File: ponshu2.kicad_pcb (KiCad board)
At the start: 2 copper layers, 61.6 x 41.7 mm, 58 parts, among them J1 Conn_01x04, J10 Conn_01x01, J11 Conn_01x01, J12 Conn_01x01, J13 Conn_01x01, J14 Conn_01x01, J15 Conn_01x01, J16 Conn_01x01, J17 Conn_01x01, J18 Conn_01x01, J19 Conn_01x01, J2 Conn_01x01, J20 Conn_01x01, J21 Conn_01x01, J22 Conn_01x01, J23 Conn_01x01, J24 Conn_01x01, J25 Conn_01x01, J26 Conn_01x01, J27 Conn_01x02, J28 Conn_01x03, J29 Conn_01x01, J3 Conn_01x01, J30 Conn_01x01, J31 Conn_01x01, J32 Conn_01x01, J33 Conn_01x01, J34 Conn_01x01, J35 Conn_01x01, J36 Conn_01x01, J37 Conn_01x01, J38 Conn_01x01, J39 Conn_01x01, J4 Conn_01x01, J5 Conn_01x01, J6 Conn_01x01, J7 Conn_01x01, J8 Conn_01x01, J9 Conn_01x01, SW1 TS-1187A-B-A-B, SW2 TS-1187A-B-A-B, U1 XC6206P332MR, U2 STM32F072CBT6

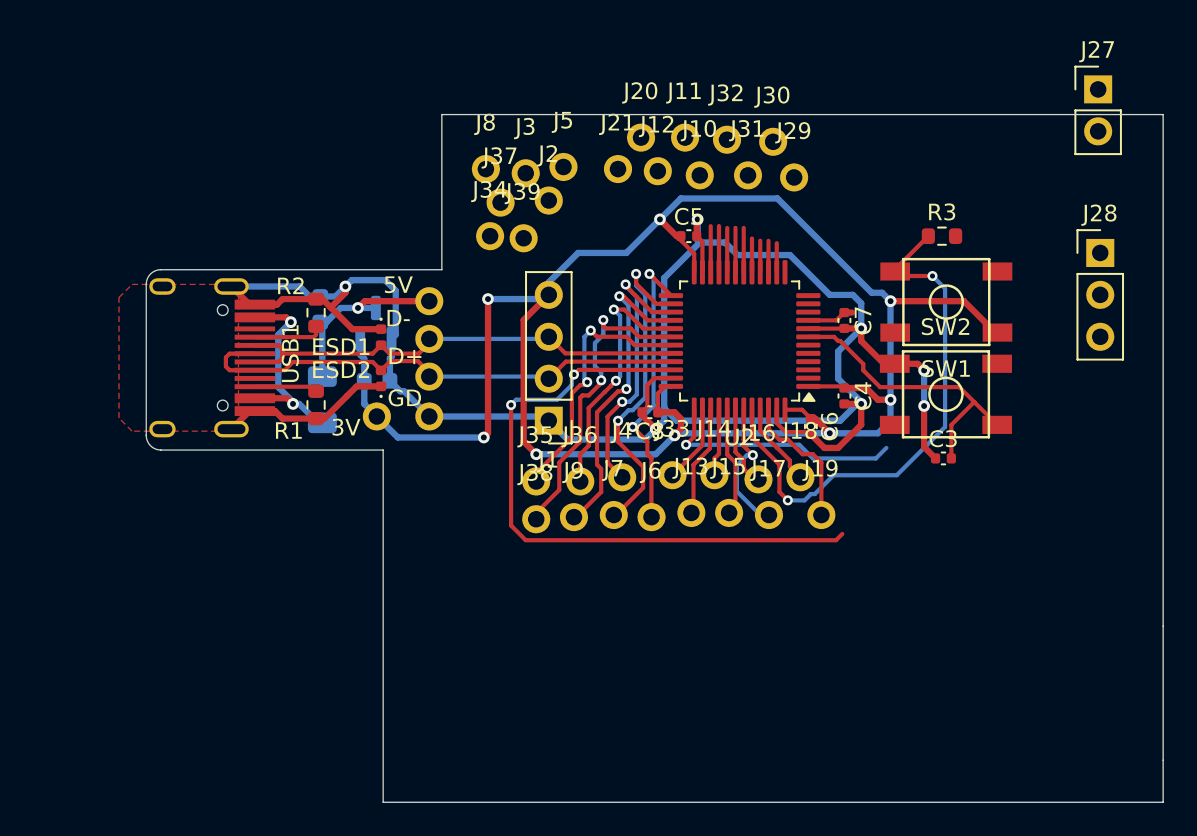
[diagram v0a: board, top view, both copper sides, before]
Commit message: kiban no ana kankaku hiroku shita
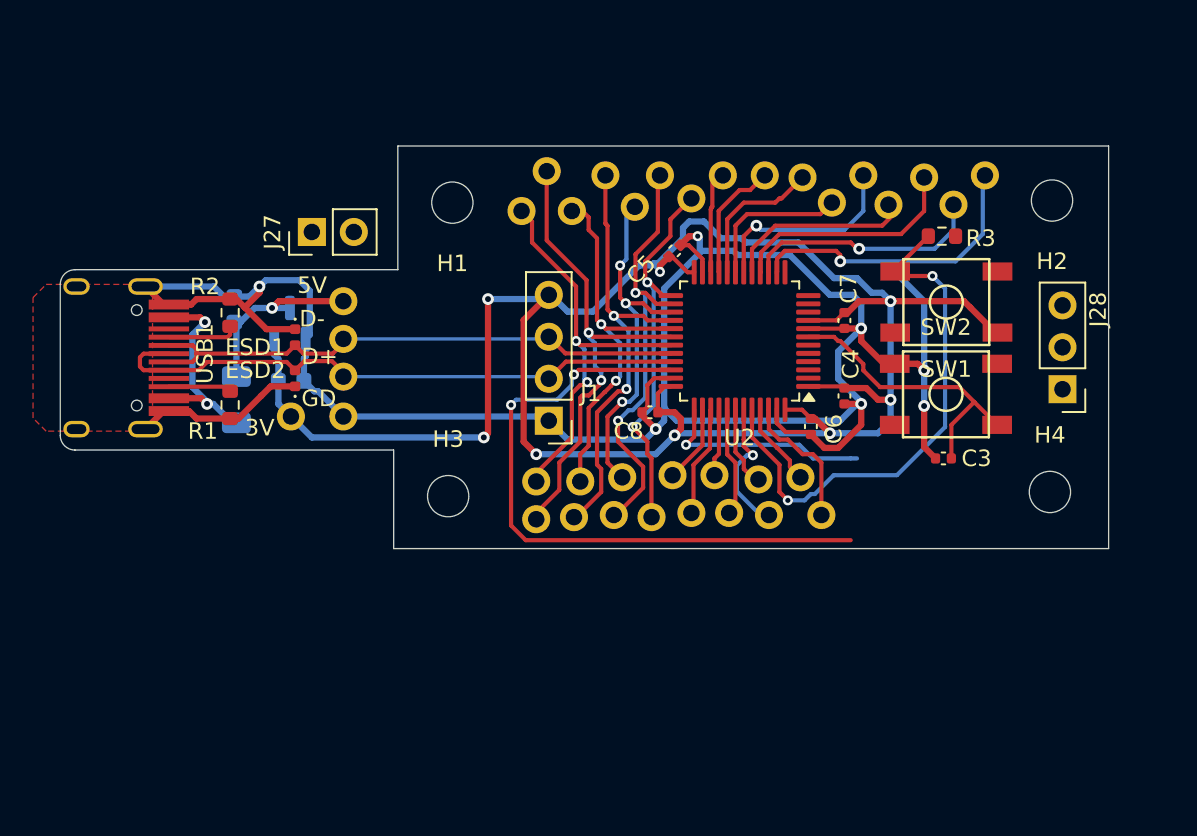
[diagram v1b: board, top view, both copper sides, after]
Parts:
- added H1: MountingHole, MountingHole:MountingHole_2.5mm, F.Cu at (77.1, 67.3)
- added H2: MountingHole, MountingHole:MountingHole_2.5mm, F.Cu at (113.4, 67.2)
- added H3: MountingHole, MountingHole:MountingHole_2.5mm, F.Cu at (76.8, 85.1)
- added H4: MountingHole, MountingHole:MountingHole_2.5mm, F.Cu at (113.3, 84.8)
- moved J27 48.4 mm to (68.6, 69.1), turned to 90 degrees
- moved J30 11.6 mm to (107.4, 67.4)
- moved J29 11.6 mm to (109.3, 65.7)
- moved J31 10.7 mm to (105.7, 65.8)
- moved J32 10.5 mm to (103.5, 67.4)
- moved J10 9.91 mm to (102.0, 65.7)
- moved J11 9.72 mm to (100.1, 67.3)
- moved J12 8.77 mm to (98.3, 65.8)
- moved J28 8.57 mm to (114.0, 78.6), turned to 180 degrees
- moved J5 7.98 mm to (91.6, 67.1)
- moved J20 7.83 mm to (96.0, 65.7)
- moved J8 7.25 mm to (86.4, 65.7)
- moved J3 6.91 mm to (88.1, 67.6)
- moved J2 6.90 mm to (89.7, 65.7)
- moved J21 6.36 mm to (93.5, 65.7)
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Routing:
- net Net-(J29-Pin_1): track 1.76 -> 18.3 mm, vias 0 -> 1
- net Net-(J30-Pin_1): track 1.91 -> 14.7 mm, vias 0 -> 1
- net Net-(J31-Pin_1): track 1.91 -> 14.2 mm
- net GND: track 134.6 -> 145.2 mm
- net Net-(J38-Pin_1): track 19.0 -> 29.4 mm
- net Net-(J10-Pin_1): track 2.69 -> 12.4 mm, vias 0 -> 1
- net Net-(J32-Pin_1): track 2.05 -> 11.6 mm
- net Net-(J34-Pin_1): track 16.0 -> 25.3 mm
- net Net-(J8-Pin_1): track 19.5 -> 27.5 mm
- net Net-(J36-Pin_1): track 15.5 -> 23.3 mm
- net +3.3V: track 119.1 -> 126.2 mm
- net Net-(J11-Pin_1): track 2.69 -> 9.24 mm
- net Net-(J12-Pin_1): track 2.68 -> 8.82 mm
- net Net-(J2-Pin_1): track 20.3 -> 26.4 mm
- net Net-(J5-Pin_1): track 17.7 -> 23.4 mm
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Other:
- board size 61.6 x 41.7 mm -> 63.5 x 24.4 mm
